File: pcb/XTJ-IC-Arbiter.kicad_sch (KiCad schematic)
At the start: 58 parts, among them IC1 TLV3704IN, J3 DTM13-12PA-R008, U1 LM2675N-5.0/NOPB, U2 CDP68HC68S1, U3 EEC-325X4A, U4 MCP2562-H-P, U5 SP723APP, U6 MCP1700-3302E/TO, U7 DS18B20

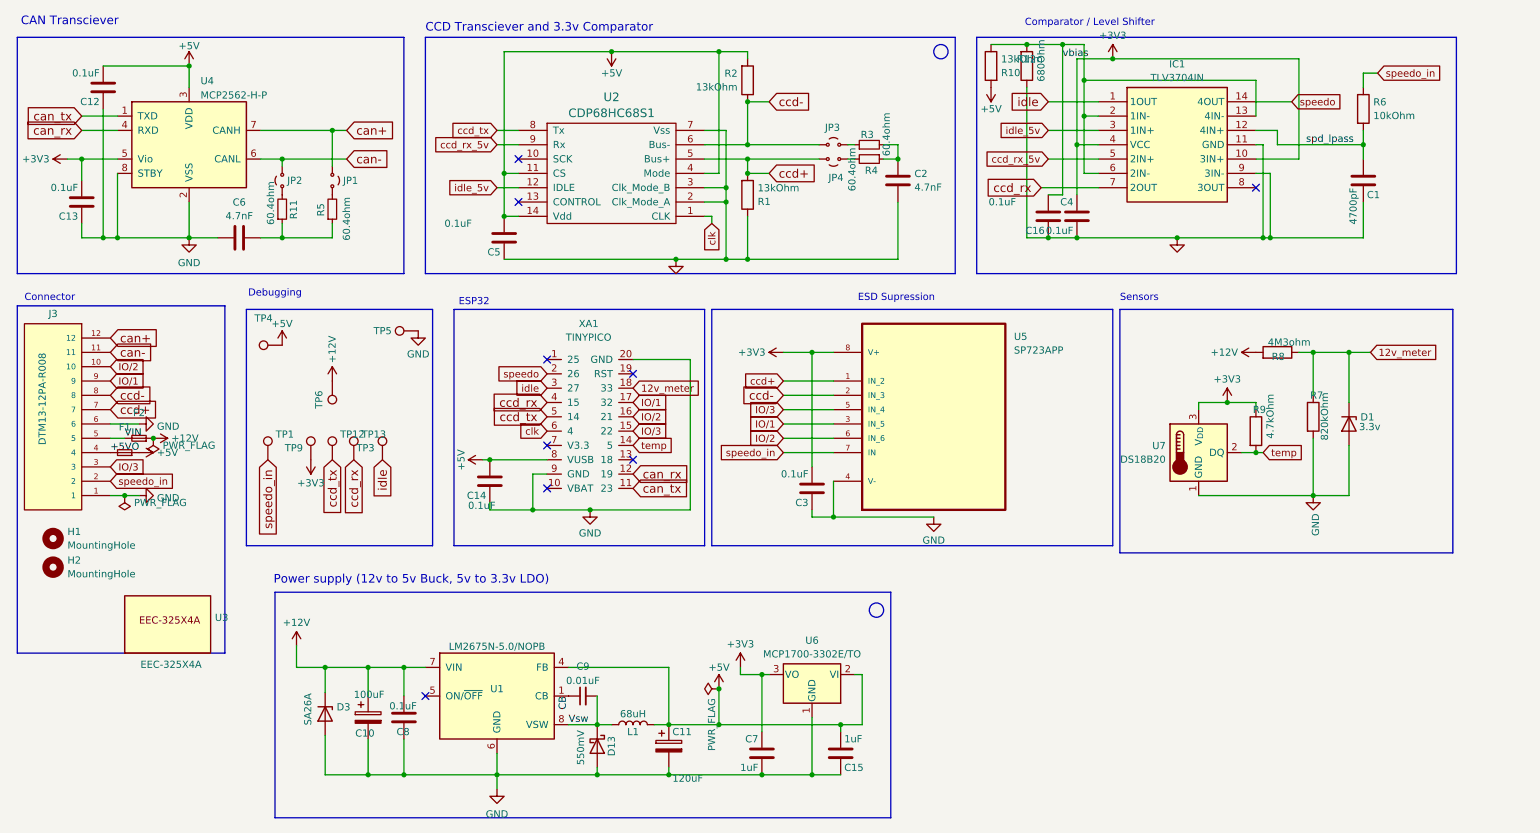
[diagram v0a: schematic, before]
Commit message: wip
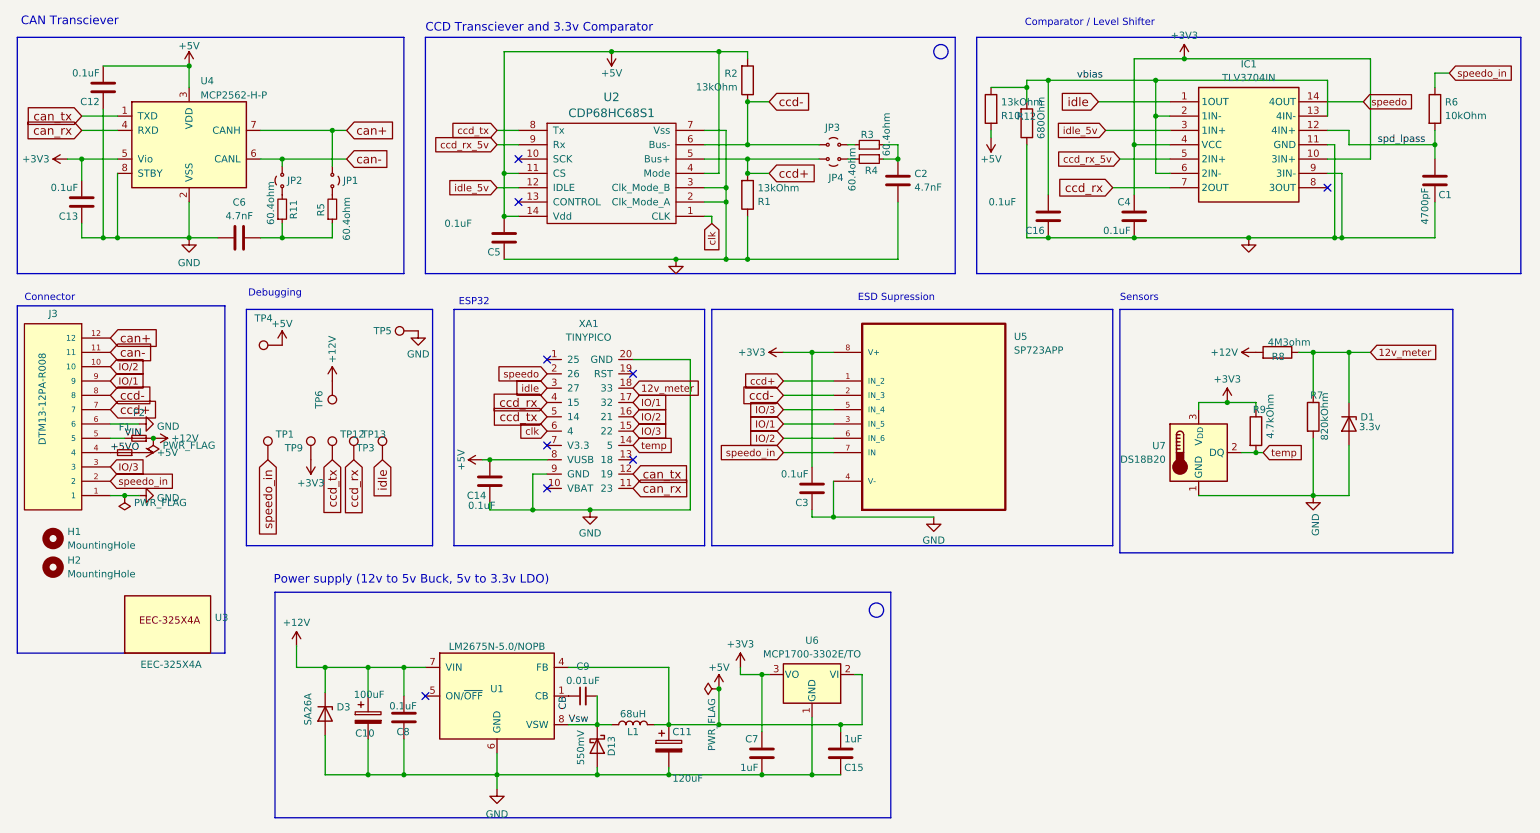
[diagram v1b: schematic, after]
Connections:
- net can_rx: now also XA1.11 (23); no longer XA1.12 (19)
- net can_tx: now also XA1.12 (19); no longer XA1.11 (23)
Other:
- moved on the sheet: C1, C4, IC1, R10, R12, R6
